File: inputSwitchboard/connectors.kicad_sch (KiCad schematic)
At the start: 11 parts, among them J3 INPUT SEL, J4 OUTPUT SEL, J5 INT CTRL, J6 EXT CTRL, J7 NES, J8 GPIO, J9 GPIO-ADC

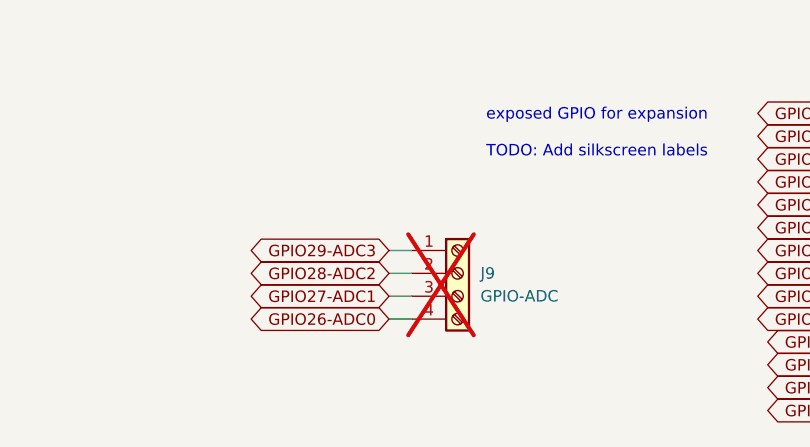
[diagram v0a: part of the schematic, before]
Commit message: finished routing
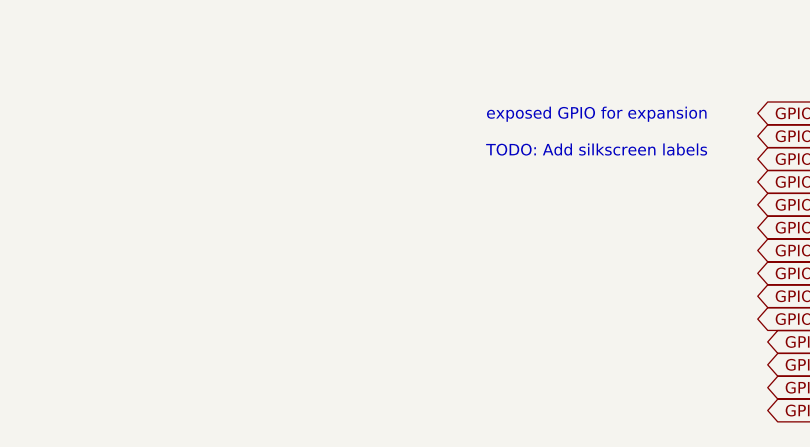
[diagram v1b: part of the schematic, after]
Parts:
- removed J9: GPIO-ADC, TerminalBlock:TerminalBlock_MaiXu_MX126-5.0-04P_1x04_P5.00mm, symbol Connector:Screw_Terminal_01x04
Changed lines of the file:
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@@
-	(wire
-		(pts
-			(xy 185.42 120.65) (xy 182.88 120.65)
-		)
-		(stroke
-			(width 0)
-			(type default)
-		)
-	)
 	(wire
 		(pts
@@
 	(wire
 		(pts
-			(xy 185.42 123.19) (xy 182.88 123.19)
-		)
-		(stroke
-			(width 0)
-			(type default)
-		)
-	)
-	(wire
-		(pts
 			(xy 149.86 62.23) (xy 157.48 62.23)
 		)
@@
 	(wire
 		(pts
-			(xy 185.42 118.11) (xy 182.88 118.11)
-		)
-		(stroke
-			(width 0)
-			(type default)
-		)
-	)
-	(wire
-		(pts
 			(xy 234.95 77.47) (xy 237.49 77.47)
 		)
@@
 		(pts
 			(xy 69.85 62.23) (xy 77.47 62.23)
-		)
-		(stroke
-			(width 0)
-			(type default)
-		)
-	)
-	(wire
-		(pts
-			(xy 185.42 125.73) (xy 182.88 125.73)
 		)
 		(stroke
@@
 		)
 	)
-	(global_label "GPIO29-ADC3"
-		(shape bidirectional)
-		(at 182.88 118.11 180)
-		(fields_autoplaced yes)
-		(effects
-			(font
-				(size 1.27 1.27)
-			)
-			(justify right)
-		)
-		(property "Intersheetrefs" "${INTERSHEET_REFS}"
-			(at 165.4787 118.11 0)
-			(effects
-				(font
-					(size 1.27 1.27)
-				)
-				(justify right)
-				(hide yes)
-			)
-		)
-	)
 	(global_label "GPIO15"
 		(shape bidirectional)
@@
 		)
 	)
-	(global_label "GPIO26-ADC0"
-		(shape bidirectional)
-		(at 182.88 125.73 180)
-		(fields_autoplaced yes)
-		(effects
-			(font
-				(size 1.27 1.27)
-			)
-			(justify right)
-		)
-		(property "Intersheetrefs" "${INTERSHEET_REFS}"
-			(at 165.4787 125.73 0)
-			(effects
-				(font
-					(size 1.27 1.27)
-				)
-				(justify right)
-				(hide yes)
-			)
-		)
-	)
 	(global_label "CTRL-INT-5-D3"
 		(shape output)
@@
 		)
 	)
-	(global_label "GPIO28-ADC2"
-		(shape bidirectional)
-		(at 182.88 120.65 180)
-		(fields_autoplaced yes)
-		(effects
-			(font
-				(size 1.27 1.27)
-			)
-			(justify right)
-		)
-		(property "Intersheetrefs" "${INTERSHEET_REFS}"
-			(at 165.4787 120.65 0)
-			(effects
-				(font
-					(size 1.27 1.27)
-				)
-				(justify right)
-				(hide yes)
-			)
-		)
-	)
 	(global_label "PROC-NES-4-VCC"
 		(shape input)
@@
 		(property "Intersheetrefs" "${INTERSHEET_REFS}"
 			(at 130.6068 85.09 0)
-			(effects
-				(font
-					(size 1.27 1.27)
-				)
-				(justify right)
-				(hide yes)
-			)
-		)
-	)
-	(global_label "GPIO27-ADC1"
-		(shape bidirectional)
-		(at 182.88 123.19 180)
-		(fields_autoplaced yes)
-		(effects
-			(font
-				(size 1.27 1.27)
-			)
-			(justify right)
-		)
-		(property "Intersheetrefs" "${INTERSHEET_REFS}"
-			(at 165.4787 123.19 0)
 			(effects
 				(font
@@
 					(unit 1)
 				)
-			)
-		)
-	)
-	(symbol
-		(lib_id "Connector:Screw_Terminal_01x04")
-		(at 190.5 120.65 0)
-		(unit 1)
-		(exclude_from_sim no)
-		(in_bom no)
-		(on_board yes)
-		(dnp yes)
-		(fields_autoplaced yes)
-		(property "Reference" "J9"
-			(at 193.04 120.6499 0)
-			(effects
-				(font
-					(size 1.27 1.27)
-				)
-				(justify left)
-			)
-		)
-		(property "Value" "GPIO-ADC"
-			(at 193.04 123.1899 0)
-			(effects
-				(font
-					(size 1.27 1.27)
-				)
-				(justify left)
-			)
-		)
-		(property "Footprint" "TerminalBlock:TerminalBlock_MaiXu_MX126-5.0-04P_1x04_P5.00mm"
-			(at 190.5 120.65 0)
-			(effects
-				(font
-					(size 1.27 1.27)
-				)
-				(hide yes)
-			)
-		)
-		(property "Datasheet" "~"
-			(at 190.5 120.65 0)
-			(effects
-				(font
-					(size 1.27 1.27)
-				)
-				(hide yes)
-			)
-		)
-		(property "Description" "Generic screw terminal, single row, 01x04, script generated (kicad-library-utils/schlib/autogen/connector/)"
-			(at 190.5 120.65 0)
-			(effects
-				(font
-					(size 1.27 1.27)
-				)
-				(hide yes)
-			)
-		)
-		(pin "3"
-		)
-		(pin "2"
-		)
-		(pin "4"
-		)
-		(pin "1"
-		)
-		(instances
-			(project ""
-				(path "/45e54069-11e8-4323-b4ab-97e83e8fb66c/8d754924-1ee4-41b7-afda-6e43d02b1969"
-					(reference "J9")
-					(unit 1)
-				)
